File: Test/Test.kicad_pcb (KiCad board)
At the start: 2 copper layers, 4 parts, among them SW1 SW_PUSH

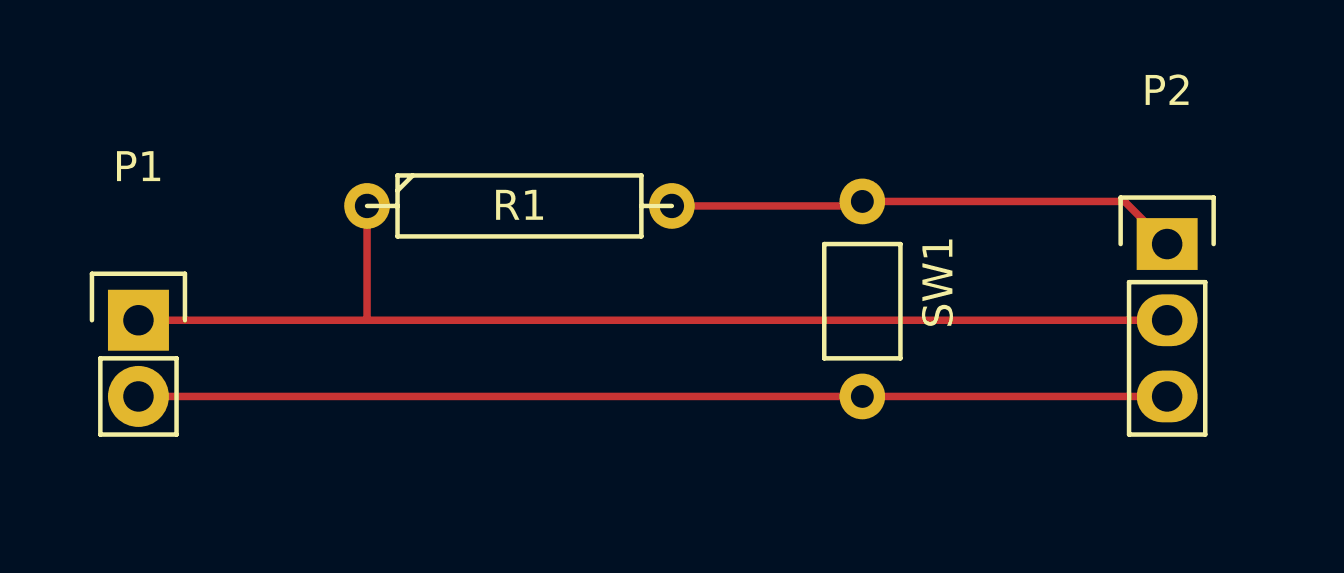
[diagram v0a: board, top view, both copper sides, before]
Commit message: Updated for Course Session 1
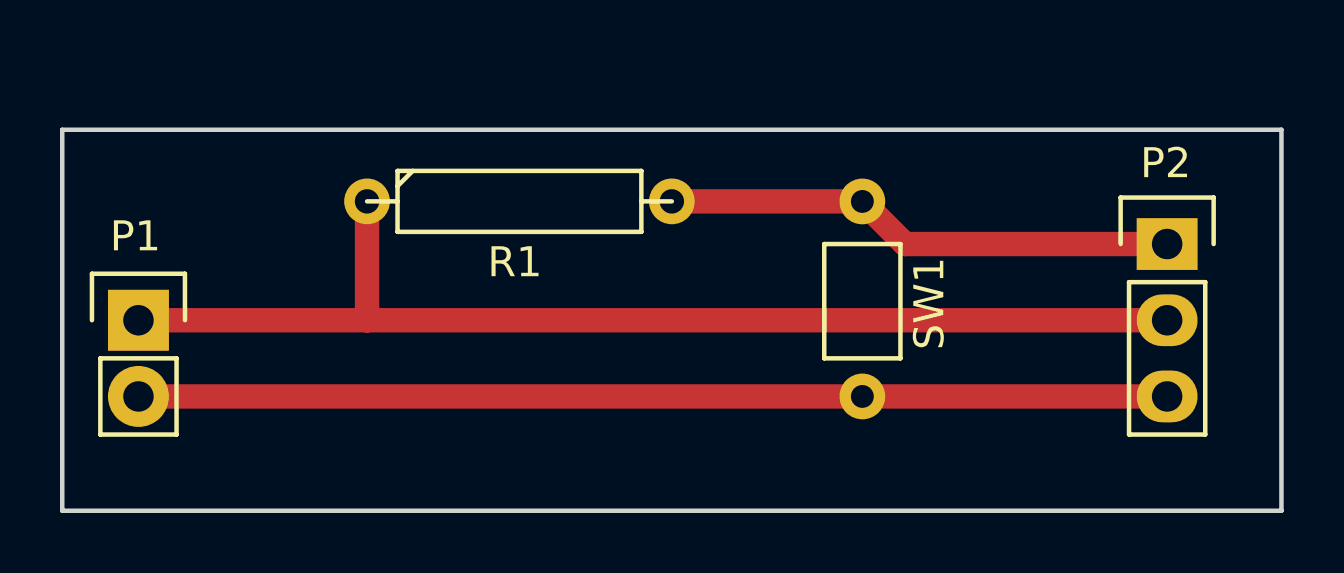
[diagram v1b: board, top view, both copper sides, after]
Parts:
- moved R1 0.15 mm to (144.8, 98.9)
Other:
- board outline added: 40.6 x 12.7 mm
- net class Default: clearance 0.2 -> 0.4826; trace_width 0.25 -> 0.8128
- rule trace_clearance: 0.2 -> 0.4826
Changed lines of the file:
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@@
-(kicad_pcb (version 4) (host pcbnew 4.0.2+e4-6225~38~ubuntu16.04.1-stable)
+(kicad_pcb (version 4) (host pcbnew 4.0.3+e1-6302~38~ubuntu16.04.1-stable)
   (general
     (links 6)
     (no_connects 0)
-    (area 0 0 0 0)
+    (area 129.464999 95.9724 170.255001 109.295001)
     (thickness 1.6)
-    (drawings 0)
+    (drawings 4)
     (tracks 9)
     (zones 0)
@@
   )
   (setup
-    (last_trace_width 0.25)
-    (trace_clearance 0.2)
+    (last_trace_width 0.8128)
+    (trace_clearance 0.4826)
     (zone_clearance 0.508)
     (zone_45_only no)
@@
     (uvia_drill 0.1)
     (uvias_allowed no)
-    (uvia_min_size 0.2)
-    (uvia_min_drill 0.1)
+    (uvia_min_size 0)
+    (uvia_min_drill 0)
     (pcb_text_width 0.3)
     (pcb_text_size 1.5 1.5)
@@
       (outputformat 1)
       (mirror false)
-      (drillshape 1)
+      (drillshape 0)
       (scaleselection 1)
-      (outputdirectory ""))
+      (outputdirectory gerbers/))
   )
   (net 0 "")
@@
   (net 3 /SW)
   (net_class Default "This is the default net class."
-    (clearance 0.2)
-    (trace_width 0.25)
+    (clearance 0.4826)
+    (trace_width 0.8128)
     (via_dia 0.6)
     (via_drill 0.4)
@@
     (descr "Through hole pin header")
     (tags "pin header")
-    (fp_text reference P1 (at 0 -5.1) (layer F.SilkS)
+    (fp_text reference P1 (at -0.1016 -2.794) (layer F.SilkS)
       (effects (font (size 1 1) (thickness 0.15)))
     )
@@
     (descr "Through hole pin header")
     (tags "pin header")
-    (fp_text reference P2 (at 0 -5.1) (layer F.SilkS)
+    (fp_text reference P2 (at -0.0508 -2.6924) (layer F.SilkS)
       (effects (font (size 1 1) (thickness 0.15)))
     )
@@
   )
   (module Discret:R4 (layer F.Cu)
-    (at 144.78 99.06)
+    (at 144.78 98.9076)
     (descr "Resitance 4 pas")
     (tags R)
-    (fp_text reference R1 (at 0 0) (layer F.SilkS)
-      (effects (font (size 1 1) (thickness 0.15)))
-    )
-    (fp_text value 10k (at 0 0) (layer F.Fab)
+    (fp_text reference R1 (at -0.1524 2.032) (layer F.SilkS)
+      (effects (font (size 1 1) (thickness 0.15)))
+    )
+    (fp_text value 10k (at -0.0508 -0.0508) (layer F.Fab)
       (effects (font (size 1 1) (thickness 0.15)))
     )
@@
   (module a-dh-libmod:SW_PUSH-2pin-6.5mm (layer F.Cu)
     (at 153.67 105.41 90)
-    (fp_text reference SW1 (at 3.81 5.08 90) (layer F.SilkS)
-      (effects (font (size 1 1) (thickness 0.15)))
-    )
-    (fp_text value SW_PUSH (at 3.81 0 90) (layer F.Fab)
+    (fp_text reference SW1 (at 3.0988 4.7752 90) (layer F.SilkS)
+      (effects (font (size 1 1) (thickness 0.15)))
+    )
+    (fp_text value SW_PUSH (at 3.81 0 90) (layer F.Fab) hide
       (effects (font (size 1 1) (thickness 0.15)))
     )
@@
       (net 3 /SW))
   )
-  (segment (start 139.7 99.06) (end 139.7 102.87) (width 0.25) (layer F.Cu) (net 1))
-  (segment (start 132.08 102.87) (end 139.7 102.87) (width 0.25) (layer F.Cu) (net 1))
-  (segment (start 139.7 102.87) (end 166.37 102.87) (width 0.25) (layer F.Cu) (net 1))
-  (segment (start 156.21 105.41) (end 166.37 105.41) (width 0.25) (layer F.Cu) (net 2))
-  (segment (start 132.08 105.41) (end 156.21 105.41) (width 0.25) (layer F.Cu) (net 2))
-  (segment (start 149.86 99.06) (end 156.06 99.06) (width 0.25) (layer F.Cu) (net 3))
+  (gr_line (start 129.54 96.52) (end 129.54 109.22) (angle 90) (layer Edge.Cuts) (width 0.15))
+  (gr_line (start 170.18 96.52) (end 129.54 96.52) (angle 90) (layer Edge.Cuts) (width 0.15))
+  (gr_line (start 170.18 109.22) (end 170.18 96.52) (angle 90) (layer Edge.Cuts) (width 0.15))
+  (gr_line (start 129.54 109.22) (end 170.18 109.22) (angle 90) (layer Edge.Cuts) (width 0.15))
+  (segment (start 139.7 98.9076) (end 139.7 102.87) (width 0.8128) (layer F.Cu) (net 1))
+  (segment (start 132.08 102.87) (end 139.7 102.87) (width 0.8128) (layer F.Cu) (net 1))
+  (segment (start 139.7 102.87) (end 166.37 102.87) (width 0.8128) (layer F.Cu) (net 1))
+  (segment (start 156.21 105.41) (end 166.37 105.41) (width 0.8128) (layer F.Cu) (net 2))
+  (segment (start 132.08 105.41) (end 156.21 105.41) (width 0.8128) (layer F.Cu) (net 2))
+  (segment (start 166.37 100.33) (end 157.63 100.33) (width 0.8128) (layer F.Cu) (net 3))
+  (segment (start 157.63 100.33) (end 156.2076 98.9076) (width 0.8128) (layer F.Cu) (net 3))
+  (segment (start 156.2076 98.9076) (end 149.86 98.9076) (width 0.8128) (layer F.Cu) (net 3))
   (segment (start 156.06 99.06) (end 156.21 98.91) (width 0.25) (layer F.Cu) (net 3))
-  (segment (start 156.21 98.91) (end 164.95 98.91) (width 0.25) (layer F.Cu) (net 3))
-  (segment (start 164.95 98.91) (end 166.37 100.33) (width 0.25) (layer F.Cu) (net 3))
 )
